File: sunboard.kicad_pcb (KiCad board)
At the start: 2 copper layers, 23 parts, among them J2 Conn_01x02, J3 Barrel_Jack, SW1 SW_Push, U1 STM32F030C8Tx, U4 MIC5209, Y1 Crystal_Small

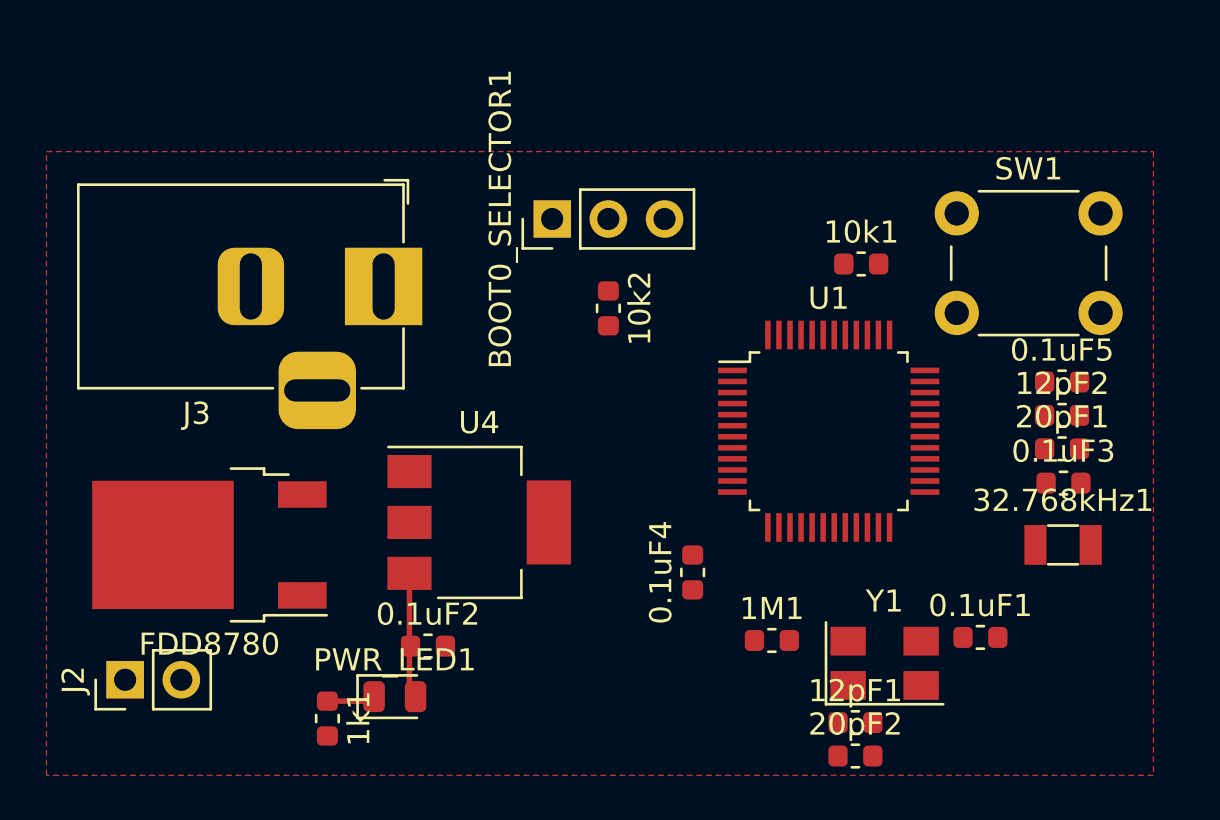
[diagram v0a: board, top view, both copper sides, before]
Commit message: some placement
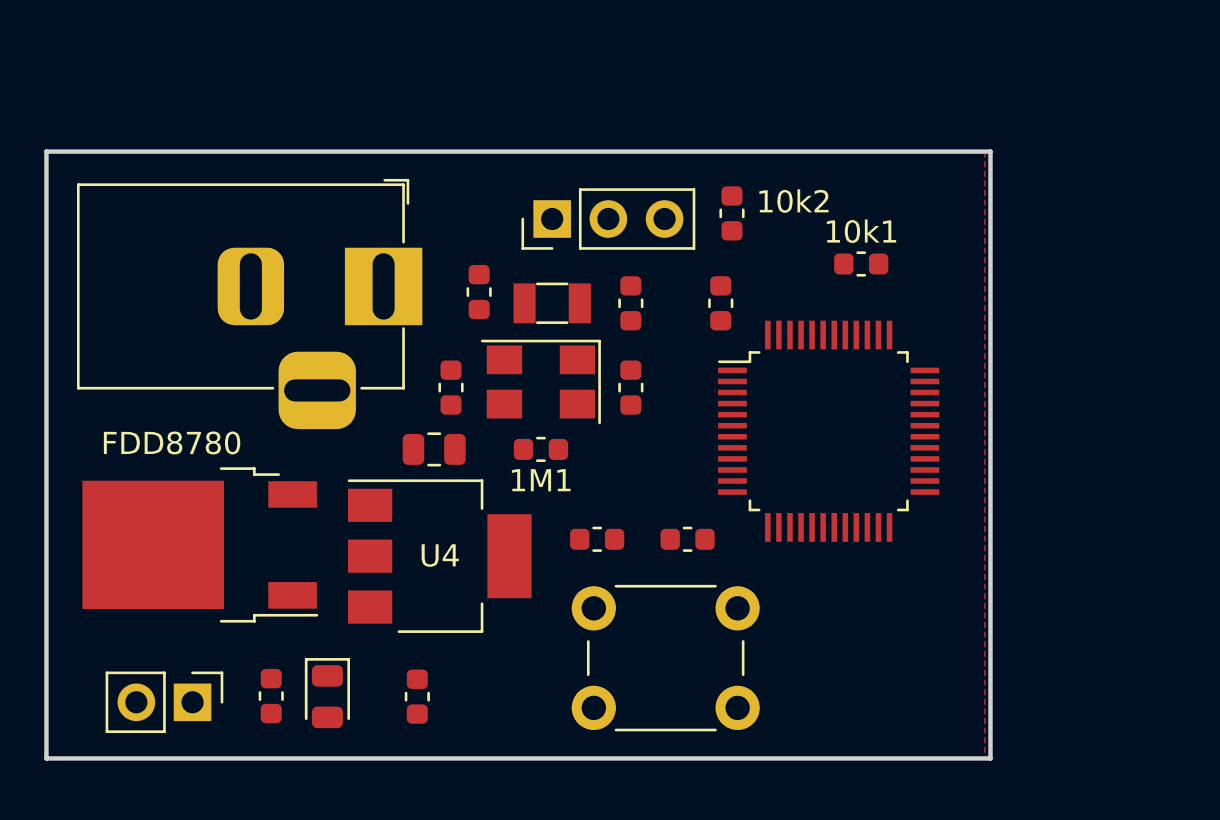
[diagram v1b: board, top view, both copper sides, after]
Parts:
- 0.1uF1: footprint Capacitor_SMD:C_0603_1608Metric -> Capacitor_SMD:C_0805_2012Metric
- moved 12pF2 26.9 mm to (61.0, 31.8), turned to 90 degrees
- moved 0.1uF1 26.1 mm to (58.9, 38.9)
- moved 32.768kHz1 25.5 mm to (64.3, 32.3)
- moved 20pF2 24.7 mm to (59.7, 36.1), turned to 90 degrees
- moved SW1 24.4 mm to (72.6, 50.5), turned to 180 degrees
- moved 0.1uF5 22.2 mm to (66.3, 42.9), turned to 180 degrees
- moved 12pF1 21.5 mm to (67.8, 32.3), turned to 90 degrees
- moved Y1 20.1 mm to (63.8, 35.8), turned to 180 degrees
- moved 20pF1 19.7 mm to (67.8, 36.1), turned to 270 degrees
- moved 0.1uF3 17.5 mm to (71.9, 32.3), turned to 90 degrees
- moved 1M1 13.5 mm to (63.8, 38.9), turned to 180 degrees
- moved 10k2 7.05 mm to (72.4, 28.2), turned to 90 degrees
- moved J2 3.21 mm to (48.0, 50.3), turned to 270 degrees
- moved PWR_LED1 3.05 mm to (54.1, 50.0), turned to 270 degrees
- moved 1k1 2.74 mm to (51.6, 50.0)
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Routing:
- net +3V3: track 5.69 -> 0.00 mm
- net Net-(1k1-Pad1): track 2.19 -> 0.00 mm
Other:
- board outline added: 42.7 x 27.4 mm
- board text added: "Sunboard Controller v1 Feb 2019"
